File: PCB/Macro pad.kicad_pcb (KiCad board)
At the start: 2 copper layers, 61 x 78 mm, 11 parts, among them J1 Conn_01x04, SW1 SW_Push, SW2 SW_Push, SW3 SW_Push, SW4 SW_Push, SW5 SW_Push, SW6 SW_Push, SW9 RotaryEncoder_Switch, U1 XIAO-RP2040-DIP

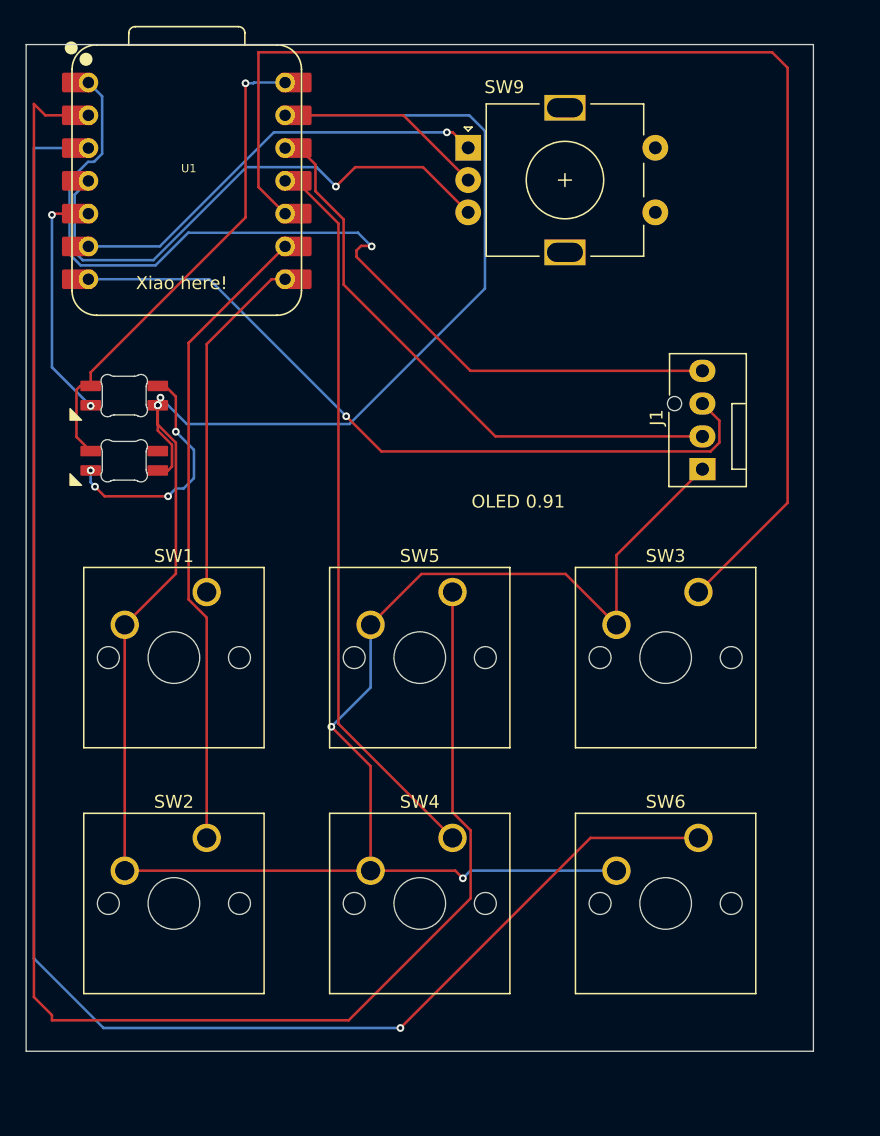
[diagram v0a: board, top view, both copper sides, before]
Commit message: Add files via upload
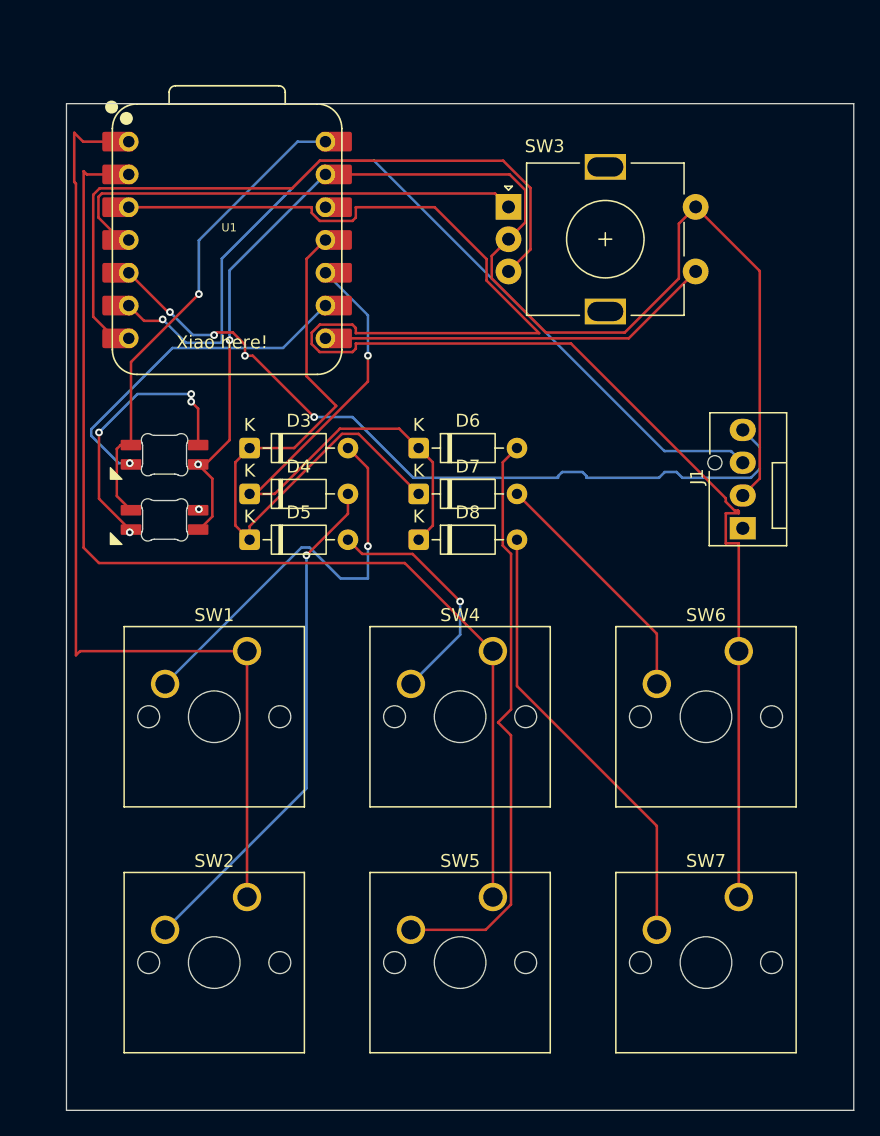
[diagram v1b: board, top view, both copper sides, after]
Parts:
- removed the SW3 at (66.1, 56.4)
- added D3: D, Diode_THT:D_DO-35_SOD27_P7.62mm_Horizontal, F.Cu at (31.3, 45.3)
- added D4: D, Diode_THT:D_DO-35_SOD27_P7.62mm_Horizontal, F.Cu at (31.3, 48.8)
- added D5: D, Diode_THT:D_DO-35_SOD27_P7.62mm_Horizontal, F.Cu at (31.3, 52.4)
- added D6: D, Diode_THT:D_DO-35_SOD27_P7.62mm_Horizontal, F.Cu at (44.4, 45.3)
- added D7: D, Diode_THT:D_DO-35_SOD27_P7.62mm_Horizontal, F.Cu at (44.4, 48.8)
- added D8: D, Diode_THT:D_DO-35_SOD27_P7.62mm_Horizontal, F.Cu at (44.4, 52.4)
- added SW7: SW_Push, Button_Switch_Keyboard:SW_Cherry_MX_1.00u_PCB, F.Cu at (69.2, 80.1)
- moved SW5 23.8 mm to (50.2, 80.1)
- moved SW6 14.8 mm to (69.2, 61.0)
- moved SW4 14.8 mm to (50.2, 61.0)
- moved SW2 5.55 mm to (31.1, 80.1)
- moved D1 5.55 mm to (24.7, 45.9)
- moved D2 5.55 mm to (24.7, 50.9)
- moved SW3 5.55 mm to (51.4, 26.6)
- moved U1 5.55 mm to (29.6, 29.1)
- moved J1 5.55 mm to (69.5, 51.5)
- moved SW1 5.55 mm to (31.1, 61.0)
- renumbered SW9 to SW3
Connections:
- net Net-(U1-GPIO28/ADC2/A2) renamed /Col2
- D1 pad 3: Net-(D1-DIN) -> /PIN_LED
- J1 pad 1: GND -> +3V3
- J1 pad 2: +3.3V -> GND
- SW1 pad 1: Net-(U1-GPIO1/RX) -> /Col0
- SW1 pad 2: GND -> Net-(D3-A)
- SW2 pad 1: Net-(U1-GPIO2/SCK) -> /Col0
- SW2 pad 2: GND -> Net-(D4-A)
- SW3 pad A: Net-(U1-GPIO7/SCL) -> /RE_A
- SW3 pad B: Net-(U1-GPIO29/ADC3/A3) -> /RE_B
- SW3 pad S1: unconnected-(SW9-PadS1) -> /PIN_RE
- SW3 pad S2: unconnected-(SW9-PadS2) -> GND
- SW4 pad 1: Net-(U1-GPIO3/MOSI) -> /Col1
- SW4 pad 2: GND -> Net-(D5-A)
- SW5 pad 1: Net-(U1-GPIO27/ADC1/A1) -> /Col1
- SW5 pad 2: GND -> Net-(D6-A)
- SW6 pad 2: GND -> Net-(D7-A)
- U1 pad 1: /SDA -> /Col0
- U1 pad 10: Net-(U1-GPIO4/MISO) -> /Row1
- U1 pad 11: Net-(U1-GPIO3/MOSI) -> /Row0
- U1 pad 2: Net-(U1-GPIO27/ADC1/A1) -> /Col1
- U1 pad 4: Net-(U1-GPIO29/ADC3/A3) -> /RE_A
- U1 pad 5: Net-(D1-DIN) -> /SDA
- U1 pad 6: Net-(U1-GPIO7/SCL) -> /SCL
- U1 pad 7: /SCL -> /RE_B
- U1 pad 8: Net-(U1-GPIO1/RX) -> /PIN_RE
- U1 pad 9: Net-(U1-GPIO2/SCK) -> /PIN_LED
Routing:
- net Net-(U1-GPIO27/ADC1/A1): track 136.8 -> 0.00 mm
- net GND: track 217.0 -> 105.8 mm, vias 5 -> 2
- net Net-(U1-GPIO4/MISO): track 98.3 -> 0.00 mm
- net /Col1: track 0.00 -> 86.9 mm
- net /Col0: track 0.00 -> 77.5 mm
- net Net-(U1-GPIO3/MOSI): track 55.9 -> 0.00 mm
- net /RE_B: track 0.00 -> 55.9 mm
- net /Row0: track 0.00 -> 49.5 mm
- net Net-(U1-GPIO2/SCK): track 49.5 -> 0.00 mm
- net /Row1: track 0.00 -> 46.4 mm, vias 0 -> 1
- net +3.3V: track 45.8 -> 0.00 mm
- net Net-(D6-A): track 0.00 -> 45.5 mm
- net Net-(U1-GPIO29/ADC3/A3): track 42.4 -> 0.00 mm, vias 1 -> 0
- net Net-(D4-A): track 0.00 -> 39.6 mm, vias 0 -> 1
- net /RE_A: track 0.00 -> 37.0 mm
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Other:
- board text removed: "OLED 0.91"
